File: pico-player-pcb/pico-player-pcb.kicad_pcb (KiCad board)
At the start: 2 copper layers, 56.9 x 66 mm, 23 parts, among them J1 AudioPlug3, U1 Pico, U2 SN76489, U3 SN76489

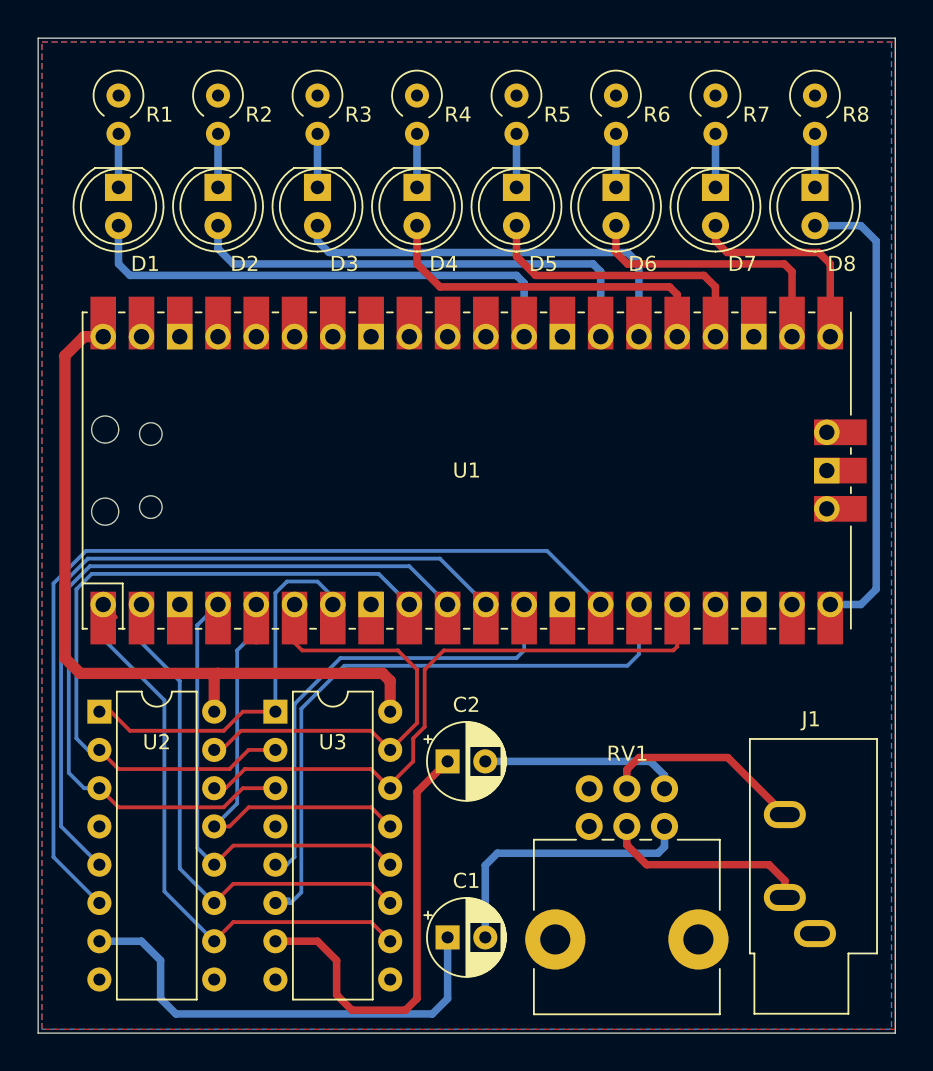
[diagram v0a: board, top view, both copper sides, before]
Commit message: minor pcb tweak
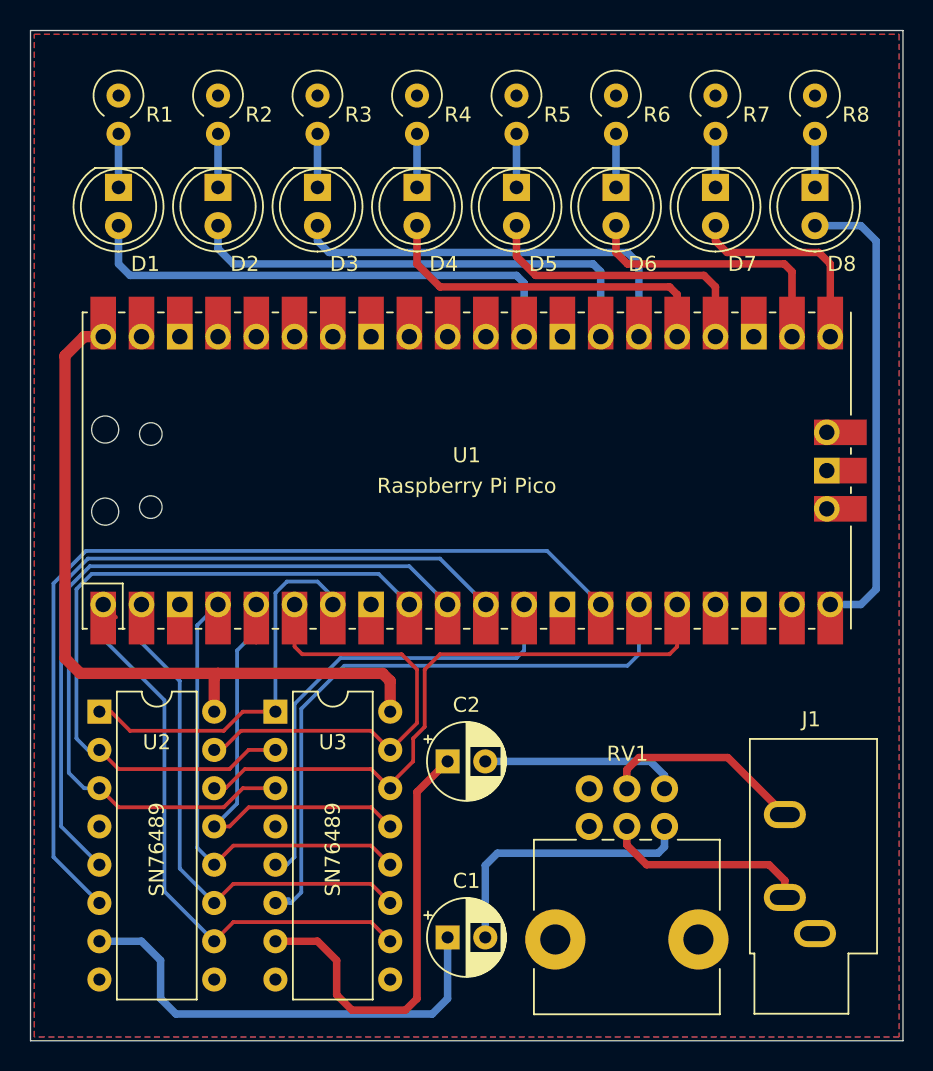
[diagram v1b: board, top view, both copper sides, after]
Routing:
- net Net-(U1-Pad6): track 30.2 -> 32.9 mm
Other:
- board size 56.9 x 66 mm -> 57.9 x 67.1 mm
- board text added: "Raspberry Pi Pico"
- board text added: "SN76489"
